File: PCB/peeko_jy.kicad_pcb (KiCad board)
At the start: 4 copper layers, 52.1 x 45.7 mm, 60 parts, among them J1 Rasberry PI Pico, J2 Conn_02x15_Odd_Even, J3 Conn_01x02_Pin, J4 Conn_01x02_Pin

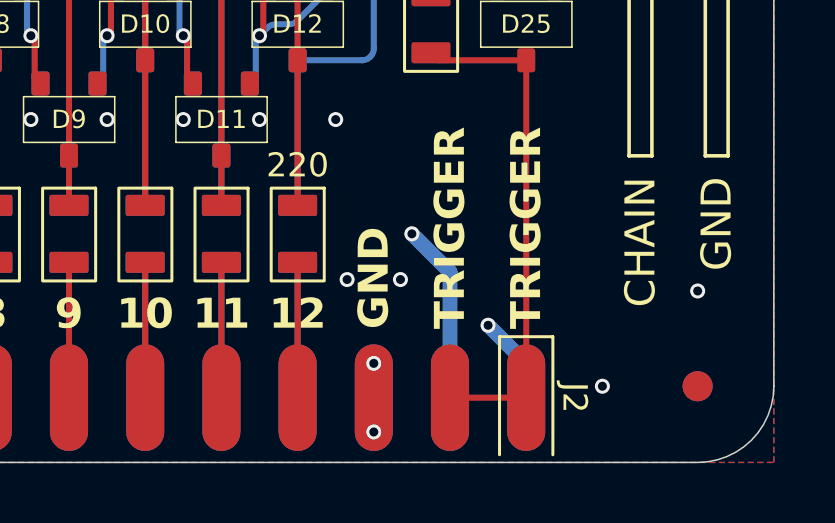
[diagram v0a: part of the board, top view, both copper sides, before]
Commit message: jy inner2 5v
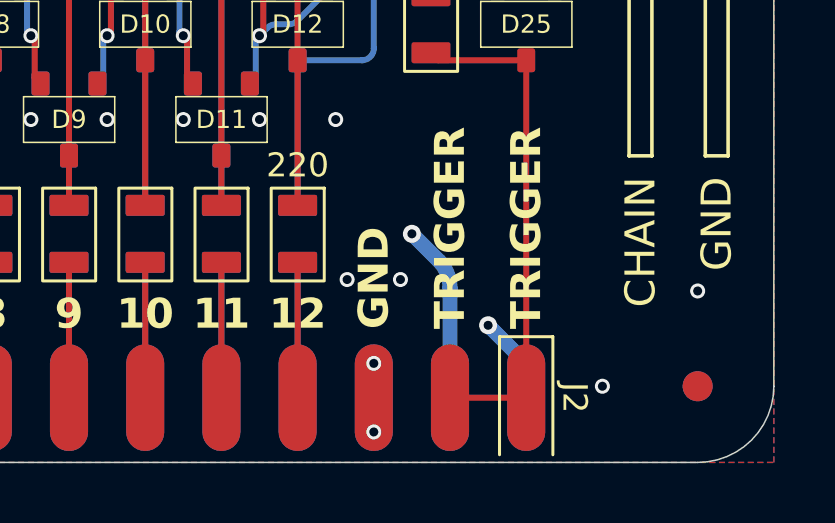
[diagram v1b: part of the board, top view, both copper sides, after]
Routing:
- net +5V: track 76.0 -> 76.5 mm
